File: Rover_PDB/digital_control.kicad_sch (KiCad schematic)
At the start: 20 parts, among them J1 Conn_01x04, J2 Conn_01x04, J3 Conn_01x04, J5 Conn_01x02, J6 Conn_01x02, J7 Conn_01x02, M1 Fan, M2 Fan, M3 Fan, Q1 NMOS, Q2 NMOS, U1 Teensy4.1, U2 MCP9808_MSOP

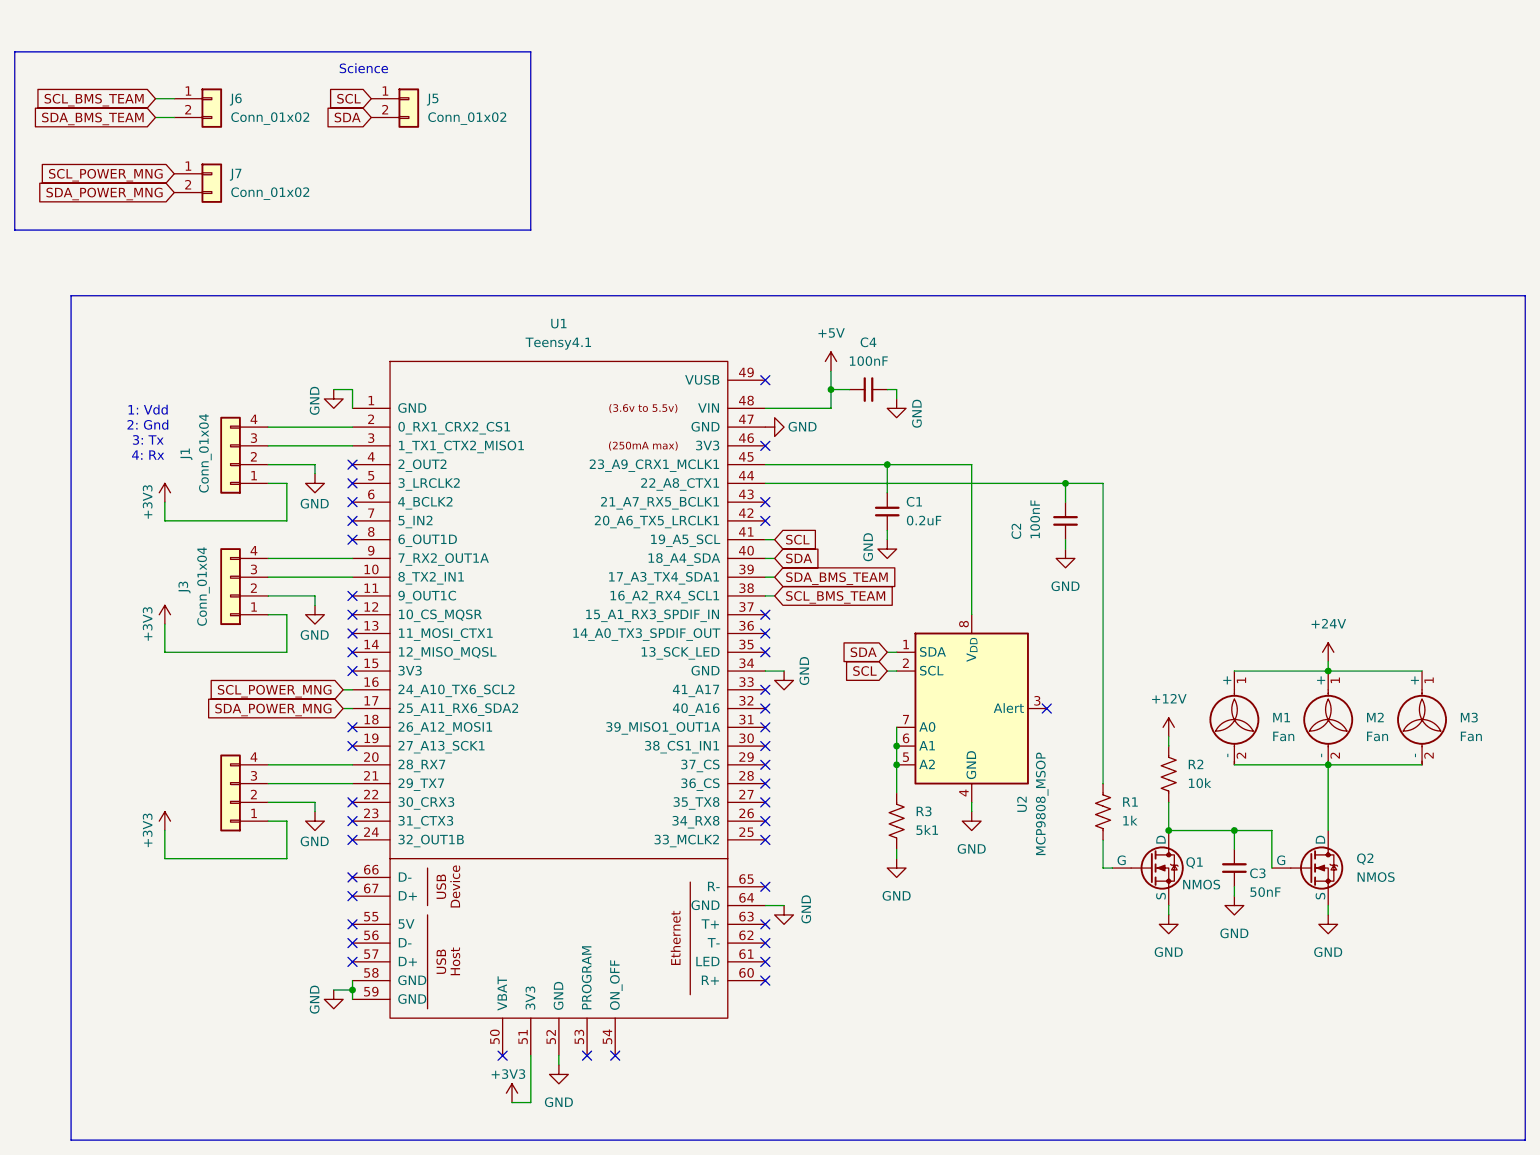
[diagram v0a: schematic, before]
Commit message: mes
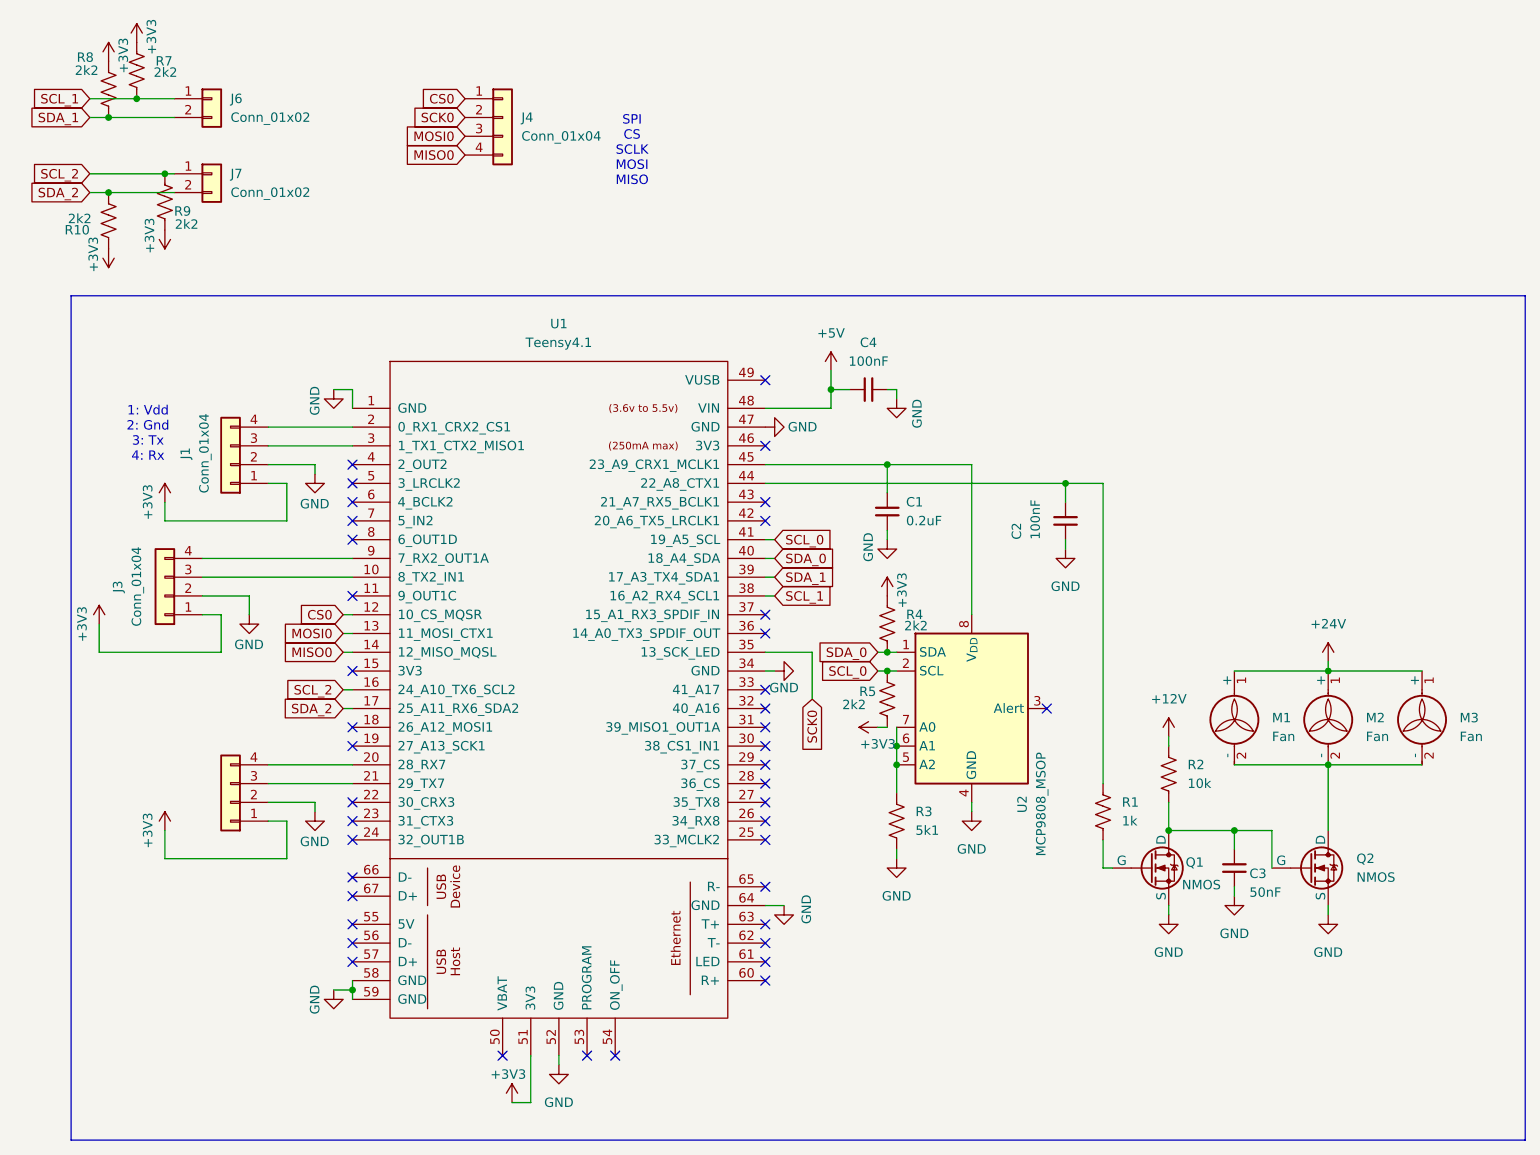
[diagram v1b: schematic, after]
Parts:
- removed J5: Conn_01x02, symbol Connector_Generic:Conn_01x02
- added J4: Conn_01x04, symbol Connector_Generic:Conn_01x04
- added R10, R4, R5, R7, R8, R9: 2k2, symbol Device:R_US
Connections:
- net +3V3: now also R10.1, R4.1, R5.1, R7.1, R8.1, R9.1
- net CS0: now reaches U1.12 (10_CS_MQSR)
- net CS0: now also J4.1 (Pin_1)
- net MOSI0: now reaches U1.13 (11_MOSI_CTX1)
- net MOSI0: now also J4.3 (Pin_3)
- net MISO0: now reaches U1.14 (12_MISO_MQSL)
- net MISO0: now also J4.4 (Pin_4)
- net SCK0: now reaches U1.35 (13_SCK_LED)
- net SCK0: now also J4.2 (Pin_2)
- net SCL renamed SCL_0
- net SCL_0: now also R5.2
- net SCL_BMS_TEAM renamed SCL_1
- net SCL_1: now also R7.2
- net SCL_POWER_MNG renamed SCL_2
- net SCL_2: now also R9.2
- net SDA renamed SDA_0
- net SDA_0: now also R4.2
- net SDA_BMS_TEAM renamed SDA_1
- net SDA_1: now also R8.2
- net SDA_POWER_MNG renamed SDA_2
- net SDA_2: now also R10.2
- no-connect marks 45 -> 41
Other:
- note added: "SPI CS SCLK MOSI MISO"
- note removed: "Science"
- moved on the sheet: J3
